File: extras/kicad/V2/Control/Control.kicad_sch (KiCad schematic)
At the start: 48 parts, among them J1 Ultrasonic Ranging, J2 Conn_01x05, J3 Output, J4 Input, J5 Conn_02x08_Top_Bottom, J6 left, J7 right, J8 UEXT_Host, P8 BeagleBone_Black_Header, P9 BeagleBone_Black_Header, U1 SparkFun-micromod, U3 LIS3DHTR, U4 BNO085-breackout, U5 TJA1042T-3, U6 PCA9557PW

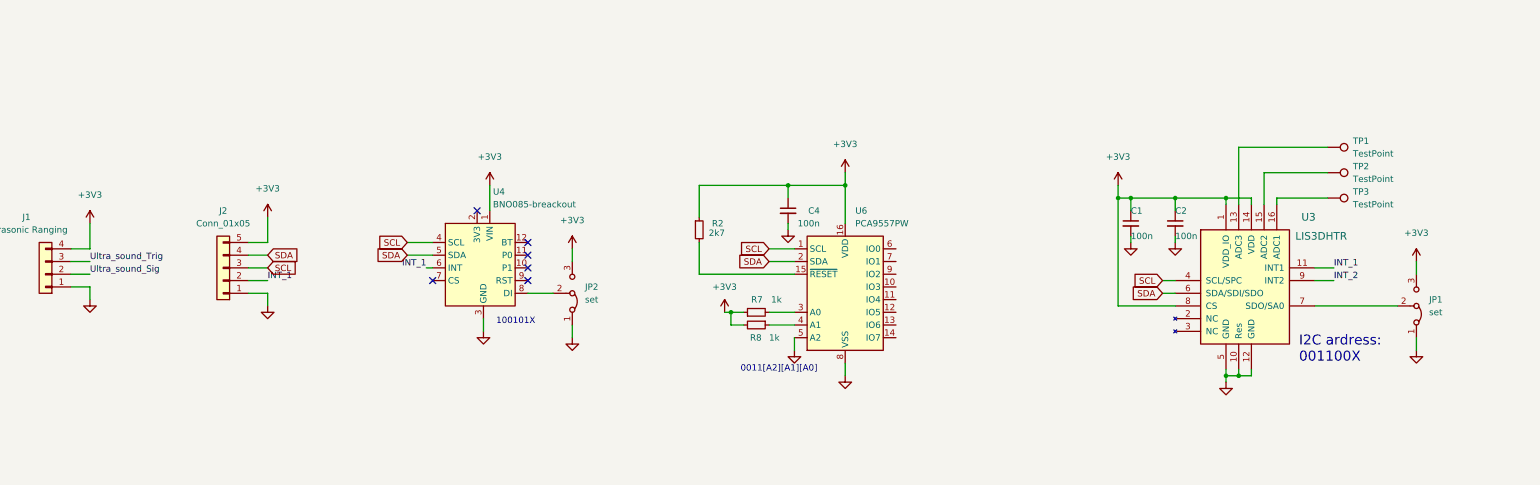
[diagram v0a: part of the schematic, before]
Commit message: y
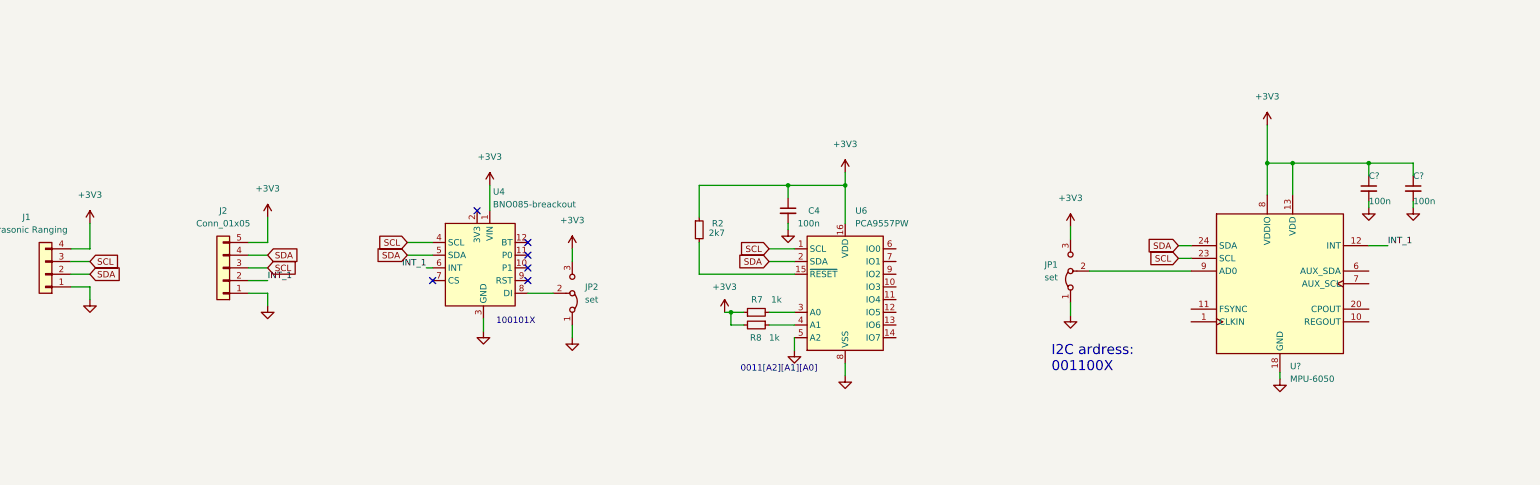
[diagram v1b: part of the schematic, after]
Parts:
- removed C1, C2: 100n, Capacitor_SMD:C_0603_1608Metric, symbol Device:C_Small
- removed TP1, TP2, TP3: TestPoint, TestPoint:TestPoint_Pad_1.5x1.5mm, symbol Connector:TestPoint
- removed U3: LIS3DHTR, digikey-footprints:VFLGA-16_3x3mm, symbol dk_Motion-Sensors-Accelerometers:LIS3DHTR
- added C? (x2): 100n, Capacitor_SMD:C_0603_1608Metric, symbol Device:C_Small
- added U?: MPU-6050, Sensor_Motion:InvenSense_QFN-24_4x4mm_P0.5mm, symbol Sensor_Motion:MPU-6050
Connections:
- net Ultra_sound_Sig is gone; now on net SDA: J1.2 (Pin_2)
- net Ultra_sound_Trig is gone; now on net SCL: J1.3 (Pin_3)
- net +3V3: now also C?.1, C?.1, U?.13 (VDD), U?.8 (VDDIO)
- net GND: now also C?.2, C?.2, U?.18 (GND)
- net INT_1: now also U?.12 (INT)
- net SCL: now also U?.23 (SCL)
- net SDA: now also U?.24 (SDA)
- net at JP1.2 (C): now also U?.9 (AD0)
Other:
- moved on the sheet: JP1
